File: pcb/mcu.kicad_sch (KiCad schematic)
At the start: 27 parts, among them SW1 PTS810, SW2 PTS810, U1 W25Q16JVSS, U2 RP2040, Y1 ABM8-272-T3

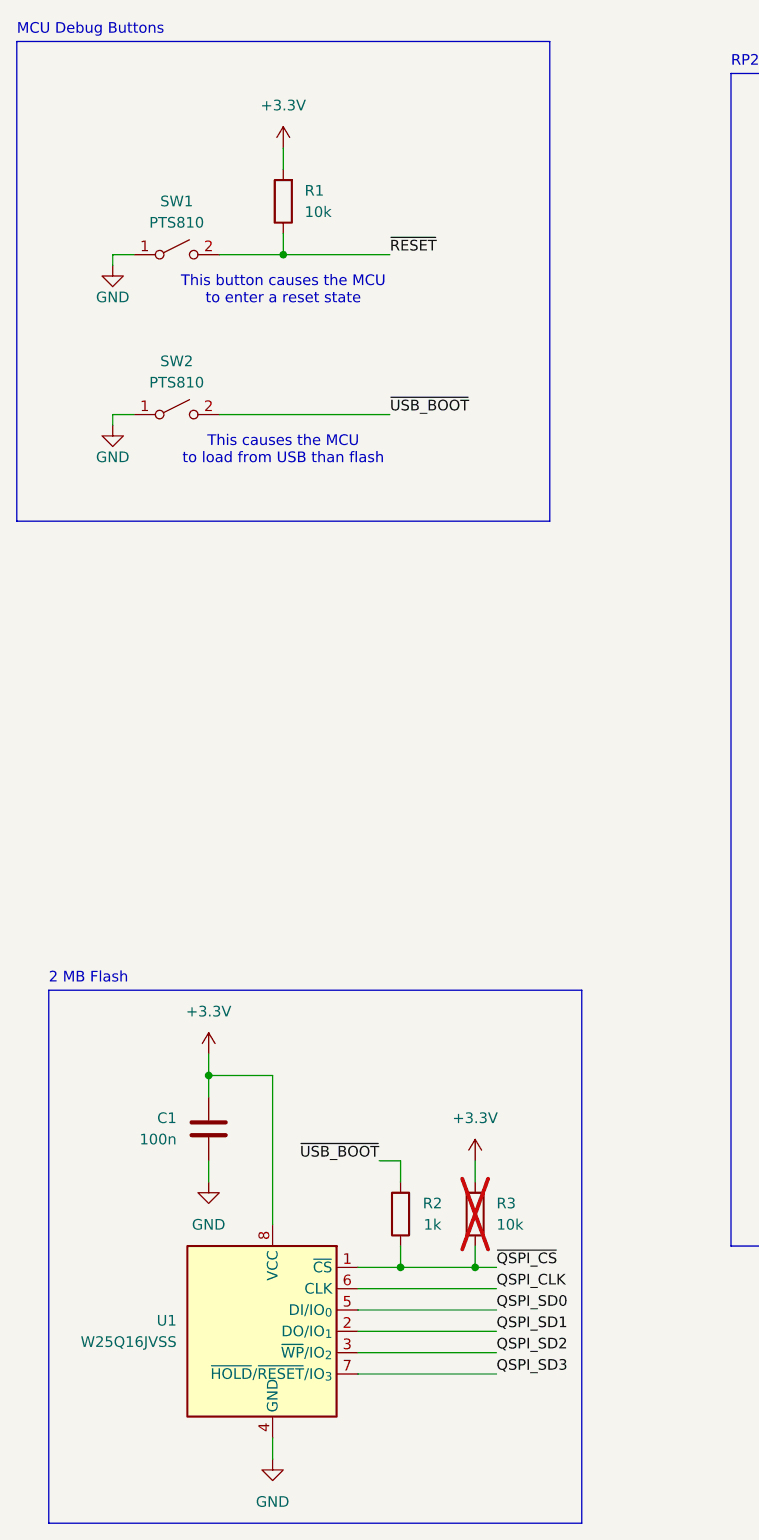
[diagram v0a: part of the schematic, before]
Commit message: cleanup routing
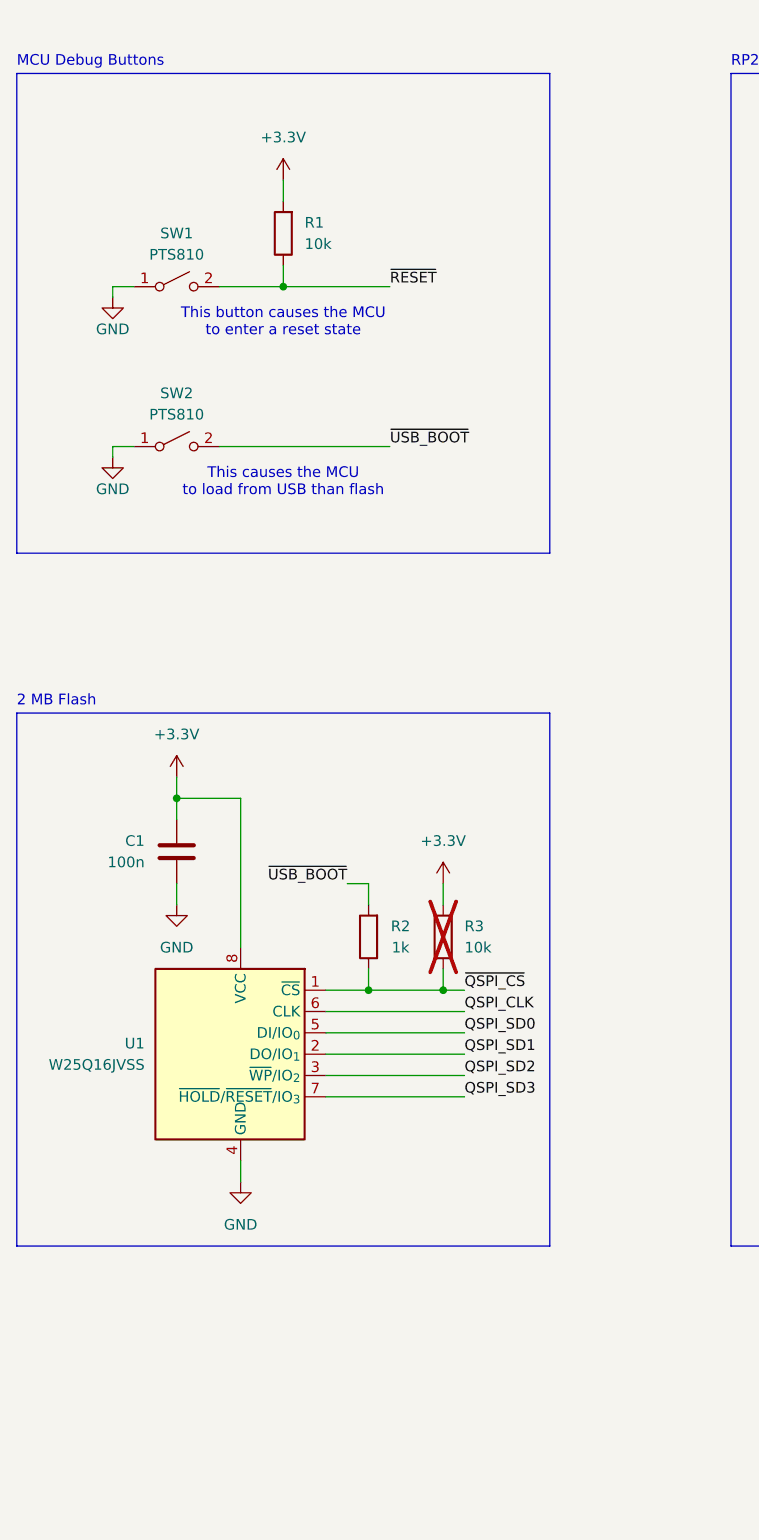
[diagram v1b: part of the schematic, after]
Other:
- moved on the sheet: C1, R1, R2, R3, SW1, SW2, U1
